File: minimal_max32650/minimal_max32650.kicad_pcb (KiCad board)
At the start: 4 copper layers, 55.9 x 45.1 mm, 105 parts, among them J1 FTSH-105-01-L-DV-K, J2 CLP-150-02-G-D-BE, Q1 50 V, Q2 50 V, U1 MX25U6432FZNI02, U2 MAXQ1065GTC+, U3 ADT75BRMZ, U4 MAX32650GCE+, U5 S80KS5122GABHM020, U6 ADP225ACPZ-R7

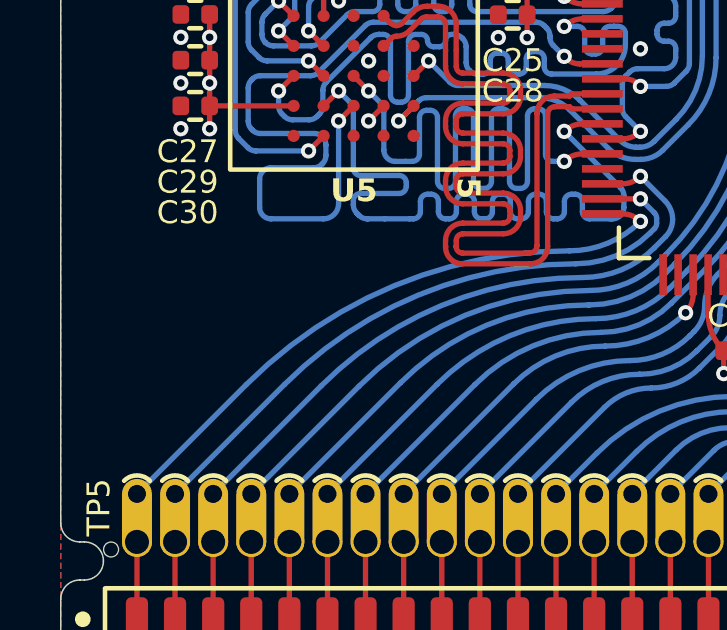
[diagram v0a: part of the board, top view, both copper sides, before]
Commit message: test workflow render
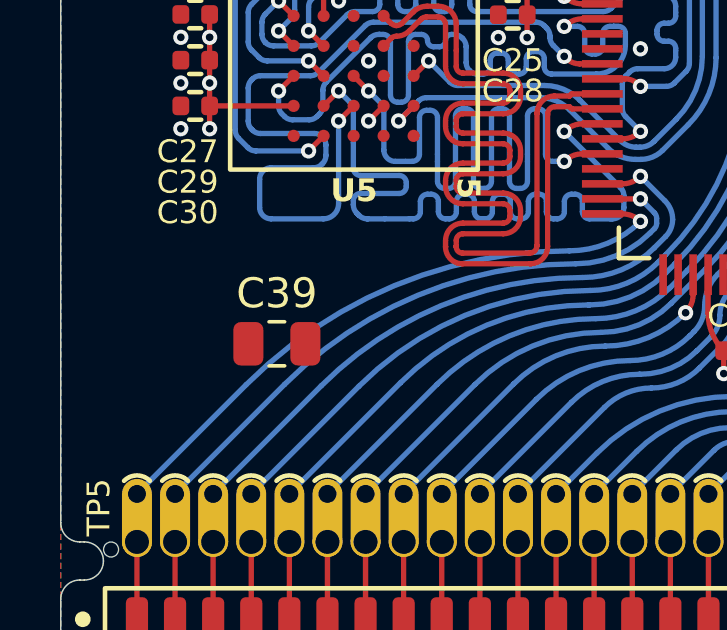
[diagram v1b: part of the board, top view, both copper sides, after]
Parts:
- added C39: C, Capacitor_SMD:C_0805_2012Metric, F.Cu at (144.2, 103.5)

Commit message: test workflow render 2
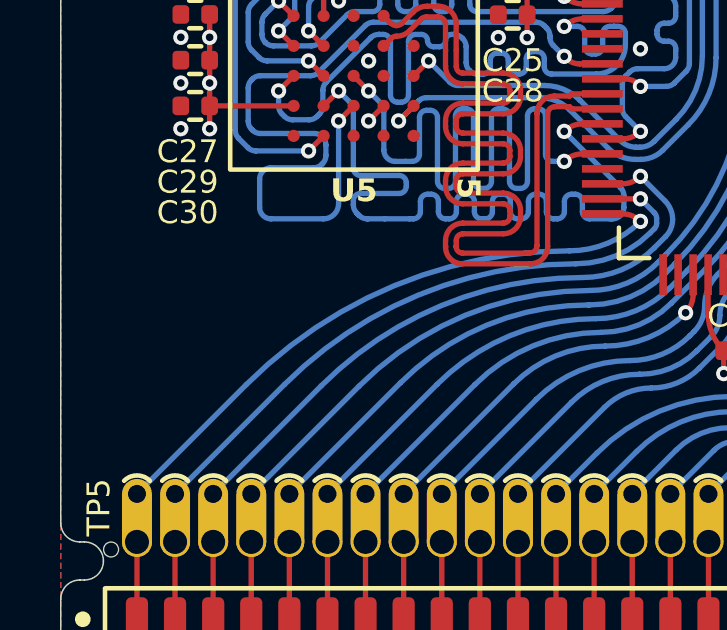
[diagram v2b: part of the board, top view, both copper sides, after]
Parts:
- removed C39: C, Capacitor_SMD:C_0805_2012Metric

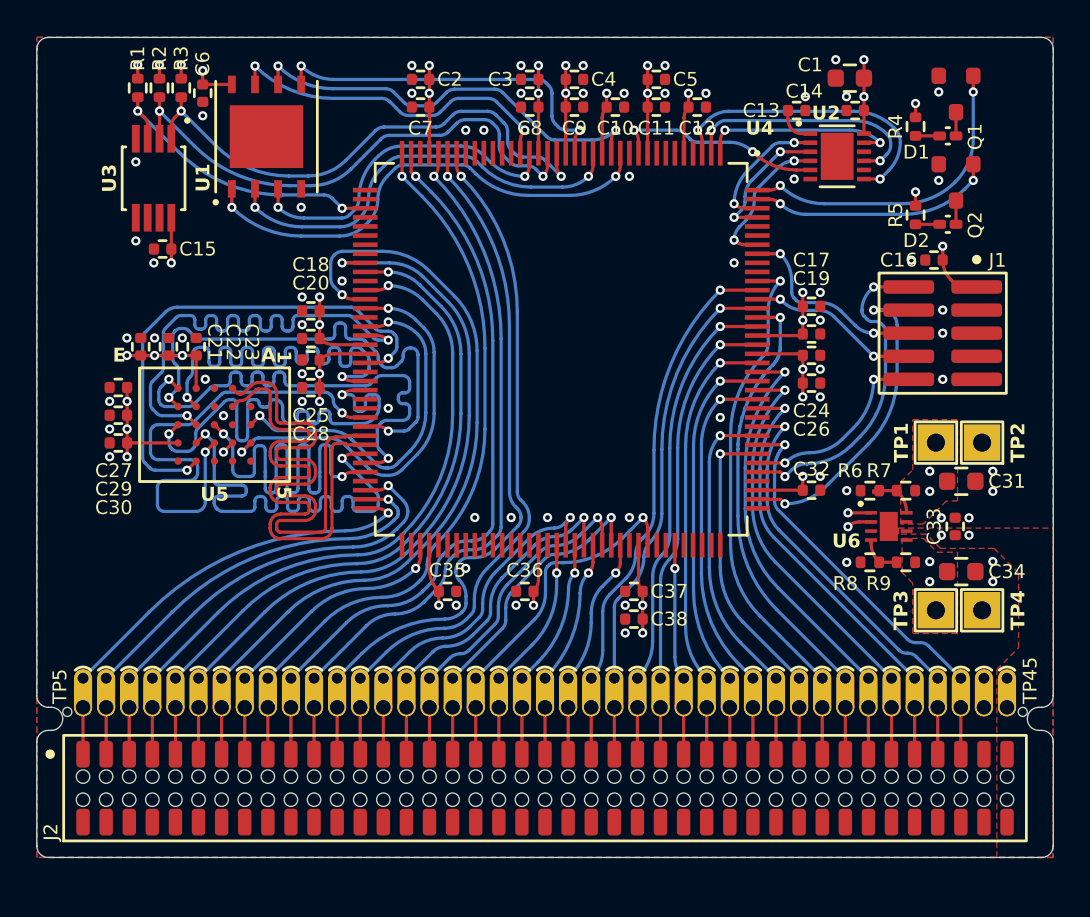
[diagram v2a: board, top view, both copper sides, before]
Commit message: development backup
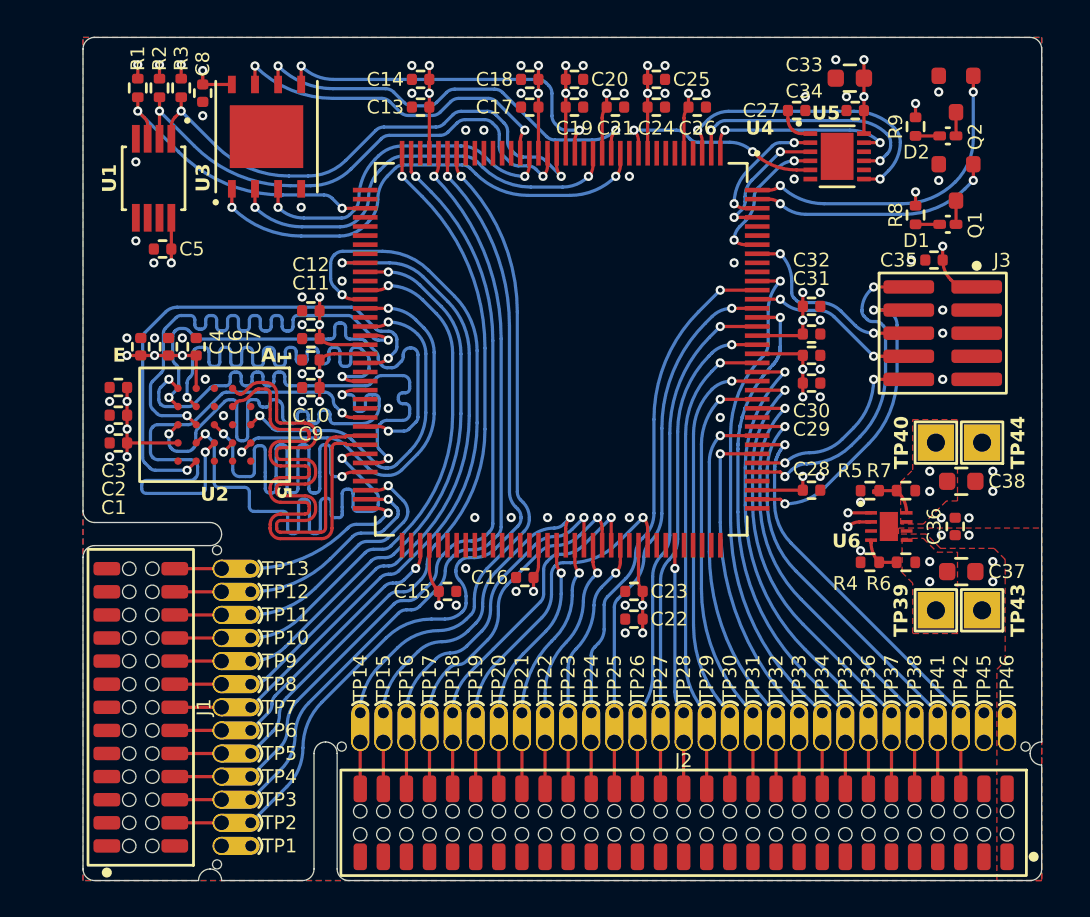
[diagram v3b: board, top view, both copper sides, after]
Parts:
- added J1: CLP-113-02-G-D-BE, connector_footprints:CLP-113-02-G-D-BE, F.Cu at (142.7, 110.1)
- added MB2: mouse-bite-50mil-1550mil, mouse_bite_footprints:mouse-bite-50mil-1550mil, F.Cu at (172.5, 112.6)
- added TP1: TestPoint, test_point_footprints:TestPoint_THTPad_Castelated, F.Cu at (147.1, 117.7)
- J2: value CLP-150-02-G-D-BE -> CLP-129-02-G-D-BE; footprint connector_footprints:CLP-141-02-G-D-BE -> connector_footprints:CLP-129-02-G-D-BE
- MB1: value mouse-bite-midle-50mil-200mil -> mouse-bite-50mil-750mil; footprint mouse_bite_footprints:mouse-bite-50mil-2138mil -> mouse_bite_footprints:mouse-bite-50mil-750mil
- moved MB1 18.4 mm to (146.5, 110.1), turned to 90 degrees
- moved TP13 10.8 mm to (147.1, 102.5), turned to 0 degrees
- moved TP2 8.98 mm to (147.1, 116.5), turned to 0 degrees
- moved TP12 8.98 mm to (147.1, 103.8), turned to 0 degrees
- moved J2 7.85 mm to (172.5, 116.5), turned to 180 degrees
- moved TP3 7.18 mm to (147.1, 115.2), turned to 0 degrees
- moved TP11 7.18 mm to (147.1, 105.0), turned to 0 degrees
- moved TP4 5.39 mm to (147.1, 113.9), turned to 0 degrees
- moved TP10 5.39 mm to (147.1, 106.3), turned to 0 degrees
- moved TP5 3.59 mm to (147.1, 112.6), turned to 0 degrees
- moved TP9 3.59 mm to (147.1, 107.6), turned to 0 degrees
- moved TP14 1.91 mm to (154.7, 112.0)
- moved TP15 1.91 mm to (156.0, 112.0)
- moved TP16 1.91 mm to (157.3, 112.0)
- moved TP17 1.91 mm to (158.5, 112.0)
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- renumbered C30 to C1, C25 to C10, C20 to C11, C18 to C12, C7 to C13, C2 to C14, C35 to C15, C36 to C16, C8 to C17, C3 to C18, C9 to C19, C29 to C2, C4 to C20, C10 to C21, C38 to C22, C37 to C23, C11 to C24, C5 to C25, C12 to C26, C13 to C27, C32 to C28, C26 to C29, C27 to C3, C24 to C30, C19 to C31, C17 to C32, C1 to C33, C14 to C34, C16 to C35, C33 to C36, C34 to C37, C31 to C38, C21 to C4, C15 to C5, C22 to C6, C23 to C7, C6 to C8, C28 to C9, D2 to D1, D1 to D2, J1 to J3, Q2 to Q1, Q1 to Q2, R8 to R4, R6 to R5, R9 to R6, R5 to R8, R4 to R9, TP8 to TP10, TP7 to TP11, TP6 to TP12, TP5 to TP13, TP17 to TP14, TP18 to TP15, TP19 to TP16, TP20 to TP17, TP21 to TP18, TP22 to TP19, TP16 to TP2, TP23 to TP20, TP24 to TP21, TP25 to TP22, TP26 to TP23, TP27 to TP24, TP28 to TP25, TP29 to TP26, TP30 to TP27, TP31 to TP28, TP32 to TP29, TP15 to TP3, TP33 to TP30, TP34 to TP31, TP35 to TP32, TP36 to TP33, TP37 to TP34, TP38 to TP35, TP39 to TP36, TP40 to TP37, TP41 to TP38, TP3 to TP39, TP14 to TP4, TP1 to TP40, TP42 to TP41, TP43 to TP42, TP4 to TP43, TP2 to TP44, TP44 to TP45, TP45 to TP46, TP13 to TP5, TP12 to TP6, TP11 to TP7, TP10 to TP8, U3 to U1, U5 to U2, U1 to U3, U2 to U5
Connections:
- J2 pad 1: /P1.25 -> /3V3
- J2 pad 10: GND -> /P2.0
- J2 pad 11: /P1.4 -> GND
- J2 pad 12: GND -> /P2.2
- J2 pad 13: /P1.6 -> GND
- J2 pad 14: GND -> /P2.4
- J2 pad 15: /P1.22 -> GND
- J2 pad 16: GND -> /P2.8
- J2 pad 17: /P0.21 -> GND
- J2 pad 18: GND -> /P2.10
- J2 pad 19: /P0.20 -> GND
- J2 pad 2: GND -> /3V3
- J2 pad 20: GND -> /P1.26
- J2 pad 21: /P0.18 -> GND
- J2 pad 22: GND -> /P1.28
- J2 pad 23: /P0.17 -> GND
- J2 pad 24: GND -> /P2.1
- J2 pad 25: /P0.16 -> GND
- J2 pad 26: GND -> /P2.3
- J2 pad 27: /P3.6 -> GND
- J2 pad 28: GND -> /P2.5
- J2 pad 29: /P1.31 -> GND
- J2 pad 3: /P1.30 -> GND
- J2 pad 30: GND -> /P0.26
- J2 pad 31: /P3.5 -> GND
- J2 pad 32: GND -> /P2.6
- J2 pad 33: /P3.7 -> GND
- J2 pad 34: GND -> /P2.7
- J2 pad 35: /P0.27 -> GND
- J2 pad 36: GND -> /P2.9
- J2 pad 37: /P3.9 -> GND
- J2 pad 38: GND -> /P2.25
- J2 pad 39: /P1.24 -> GND
- J2 pad 40: GND -> /P3.4
- J2 pad 41: /P3.8 -> GND
- J2 pad 42: GND -> /P3.8
- J2 pad 43: /P3.4 -> GND
- J2 pad 44: GND -> /P1.24
- J2 pad 45: /P2.25 -> GND
- J2 pad 46: GND -> /P3.9
- J2 pad 47: /P2.9 -> GND
- J2 pad 48: GND -> /P0.27
- J2 pad 49: /P2.7 -> GND
- J2 pad 5: /P1.23 -> GND
- J2 pad 50: GND -> /P3.7
- J2 pad 51: /P2.6 -> GND
- J2 pad 52: GND -> /P3.5
- J2 pad 53: /P0.26 -> GND
- J2 pad 54: GND -> /P1.31
- J2 pad 55: /P2.5 -> GND
- J2 pad 56: GND -> /P3.6
- J2 pad 57: /P2.3 -> GND
- J2 pad 58: GND -> /P0.16
- J2 pad 6: GND -> /P1.27
- J2 pad 7: /P1.9 -> GND
- J2 pad 8: GND -> /P1.29
- J2 pad 9: /P1.8 -> GND
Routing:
- net /P1.25: track 23.6 -> 12.3 mm
- net /P0.17: track 39.1 -> 48.5 mm
- net /P1.30: track 23.9 -> 14.4 mm
- net /P1.23: track 24.3 -> 16.6 mm
- net /P0.18: track 38.1 -> 45.5 mm
- net /P1.9: track 36.5 -> 30.6 mm
- net /P0.20: track 39.0 -> 44.5 mm
- net /P1.8: track 36.6 -> 32.5 mm
- net /P0.21: track 38.6 -> 42.0 mm
- net /P1.4: track 39.2 -> 36.9 mm
- net /P3.9: track 10.7 -> 12.9 mm
- net /P1.24: track 10.5 -> 12.7 mm
- net /P2.25: track 27.9 -> 30.0 mm
- net /P3.8: track 10.5 -> 12.6 mm
- net /P2.7: track 25.1 -> 27.1 mm
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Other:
- board size 55.9 x 45.1 mm -> 52.7 x 46.4 mm
